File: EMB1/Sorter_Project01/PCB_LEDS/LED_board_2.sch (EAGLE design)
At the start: 10 parts, among them IC1 LM358N, K2 61201021621

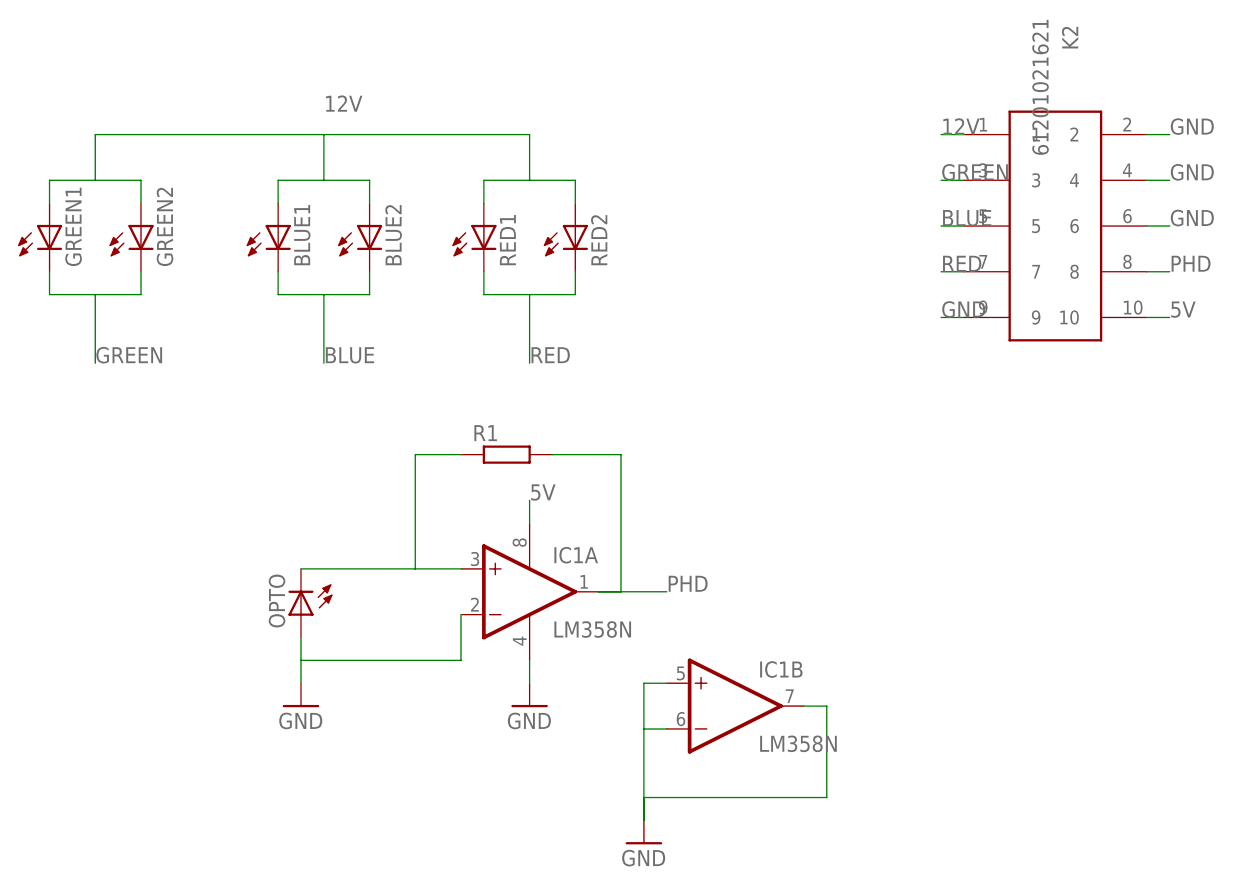
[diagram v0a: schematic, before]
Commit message: updated PCB design
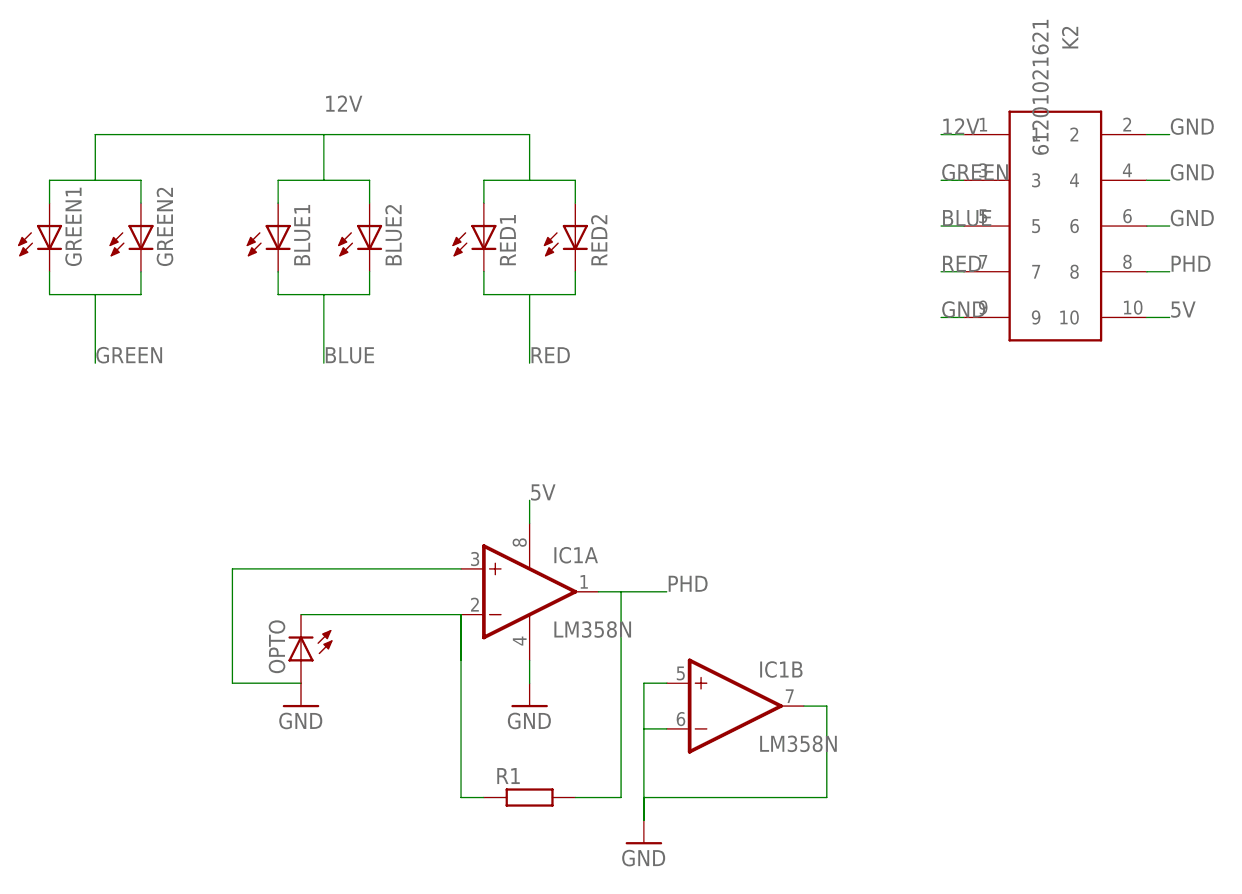
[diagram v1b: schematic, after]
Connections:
- net GND: now also IC1A.+IN; no longer IC1A.-IN
- net N$2: now also IC1A.-IN; no longer IC1A.+IN
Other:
- moved on the sheet: OPTO, R1
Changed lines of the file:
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@@
 <instance part="BLUE1" gate="G$1" x="15.24" y="83.82"/>
 <instance part="BLUE2" gate="G$1" x="25.4" y="83.82"/>
-<instance part="OPTO" gate="G$1" x="17.78" y="40.64" rot="R180"/>
+<instance part="OPTO" gate="G$1" x="17.78" y="35.56" rot="R180"/>
 <instance part="GND5" gate="1" x="17.78" y="30.48"/>
 <instance part="K2" gate="G$1" x="101.6" y="86.36" rot="R270"/>
@@
 <instance part="IC1" gate="B" x="66.04" y="30.48"/>
 <instance part="GND1" gate="1" x="43.18" y="30.48"/>
-<instance part="R1" gate="G$1" x="40.64" y="58.42"/>
+<instance part="R1" gate="G$1" x="43.18" y="20.32"/>
 <instance part="GND2" gate="1" x="55.88" y="15.24"/>
 </instances>
@@
 <nets>
 <net name="GND" class="0">
-<segment>
-<pinref part="OPTO" gate="G$1" pin="A"/>
-<pinref part="GND5" gate="1" pin="GND"/>
-<wire x1="17.78" y1="38.1" x2="17.78" y2="35.56" width="0.1524" layer="91"/>
-<pinref part="IC1" gate="A" pin="-IN"/>
-<wire x1="17.78" y1="35.56" x2="17.78" y2="33.02" width="0.1524" layer="91"/>
-<wire x1="35.56" y1="40.64" x2="35.56" y2="35.56" width="0.1524" layer="91"/>
-<wire x1="35.56" y1="35.56" x2="17.78" y2="35.56" width="0.1524" layer="91"/>
-</segment>
 <segment>
 <pinref part="K2" gate="G$1" pin="9"/>
@@
 <wire x1="111.76" y1="83.82" x2="114.3" y2="83.82" width="0.1524" layer="91"/>
 <label x="114.3" y="83.82" size="1.778" layer="95"/>
+</segment>
+<segment>
+<pinref part="GND5" gate="1" pin="GND"/>
+<pinref part="OPTO" gate="G$1" pin="A"/>
+<pinref part="IC1" gate="A" pin="+IN"/>
+<wire x1="35.56" y1="45.72" x2="10.16" y2="45.72" width="0.1524" layer="91"/>
+<wire x1="10.16" y1="45.72" x2="10.16" y2="33.02" width="0.1524" layer="91"/>
+<wire x1="10.16" y1="33.02" x2="17.78" y2="33.02" width="0.1524" layer="91"/>
 </segment>
 </net>
@@
 </segment>
 </net>
-<net name="N$2" class="0">
-<segment>
-<pinref part="OPTO" gate="G$1" pin="C"/>
-<wire x1="17.78" y1="45.72" x2="30.48" y2="45.72" width="0.1524" layer="91"/>
-<pinref part="IC1" gate="A" pin="+IN"/>
-<wire x1="30.48" y1="45.72" x2="35.56" y2="45.72" width="0.1524" layer="91"/>
-<wire x1="30.48" y1="45.72" x2="30.48" y2="58.42" width="0.1524" layer="91"/>
-<pinref part="R1" gate="G$1" pin="1"/>
-<wire x1="30.48" y1="58.42" x2="35.56" y2="58.42" width="0.1524" layer="91"/>
-</segment>
-</net>
 <net name="PHD" class="0">
 <segment>
 <pinref part="R1" gate="G$1" pin="2"/>
-<wire x1="45.72" y1="58.42" x2="53.34" y2="58.42" width="0.1524" layer="91"/>
-<wire x1="53.34" y1="58.42" x2="53.34" y2="43.18" width="0.1524" layer="91"/>
+<wire x1="48.26" y1="20.32" x2="53.34" y2="20.32" width="0.1524" layer="91"/>
+<wire x1="53.34" y1="20.32" x2="53.34" y2="43.18" width="0.1524" layer="91"/>
 <pinref part="IC1" gate="A" pin="OUT"/>
-<wire x1="53.34" y1="43.18" x2="50.8" y2="43.18" width="0.1524" layer="91"/>
-<wire x1="50.8" y1="43.18" x2="58.42" y2="43.18" width="0.1524" layer="91"/>
+<wire x1="50.8" y1="43.18" x2="53.34" y2="43.18" width="0.1524" layer="91"/>
 <label x="58.42" y="43.18" size="1.778" layer="95"/>
+<wire x1="53.34" y1="43.18" x2="58.42" y2="43.18" width="0.1524" layer="91"/>
 </segment>
 <segment>
@@
 </segment>
 </net>
+<net name="N$2" class="0">
+<segment>
+<pinref part="IC1" gate="A" pin="-IN"/>
+<wire x1="35.56" y1="40.64" x2="35.56" y2="35.56" width="0.1524" layer="91"/>
+<pinref part="OPTO" gate="G$1" pin="C"/>
+<wire x1="17.78" y1="40.64" x2="35.56" y2="40.64" width="0.1524" layer="91"/>
+<pinref part="R1" gate="G$1" pin="1"/>
+<wire x1="35.56" y1="20.32" x2="38.1" y2="20.32" width="0.1524" layer="91"/>
+<wire x1="35.56" y1="40.64" x2="35.56" y2="20.32" width="0.1524" layer="91"/>
+</segment>
+</net>
